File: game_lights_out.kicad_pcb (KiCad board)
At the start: 2 copper layers, 171.2 x 136.9 mm, 94 parts, among them SW1 SW_MEC_5E, SW10 SW_MEC_5E, SW11 SW_MEC_5E, SW12 SW_MEC_5E, SW13 SW_MEC_5E, SW14 SW_MEC_5E, SW15 SW_MEC_5E, SW16 SW_MEC_5E, SW17 SW_MEC_5E, SW18 SW_MEC_5E, SW19 SW_MEC_5E, SW2 SW_MEC_5E, SW20 SW_MEC_5E, SW21 SW_MEC_5E, SW22 SW_MEC_5E, SW23 SW_MEC_5E, SW24 SW_MEC_5E, SW25 SW_MEC_5E, SW26 SW_MEC_5E, SW27 SW_MEC_5E, SW28 SW_MEC_5E, SW29 SW_MEC_5E, SW3 SW_MEC_5E, SW30 SW_MEC_5E, SW31 SW_MEC_5E, SW32 SW_MEC_5E, SW33 SW_MEC_5E, SW34 SW_MEC_5E, SW35 SW_MEC_5E, SW36 SW_MEC_5E, SW37 SW_MEC_5E, SW38 SW_MEC_5E, SW39 SW_MEC_5E, SW4 SW_MEC_5E, SW40 SW_MEC_5E, SW5 SW_MEC_5E, SW6 SW_MEC_5E, SW7 SW_MEC_5E, SW8 SW_MEC_5E, SW9 SW_MEC_5E, U1 ATmega328-P, U2 ULN2803A

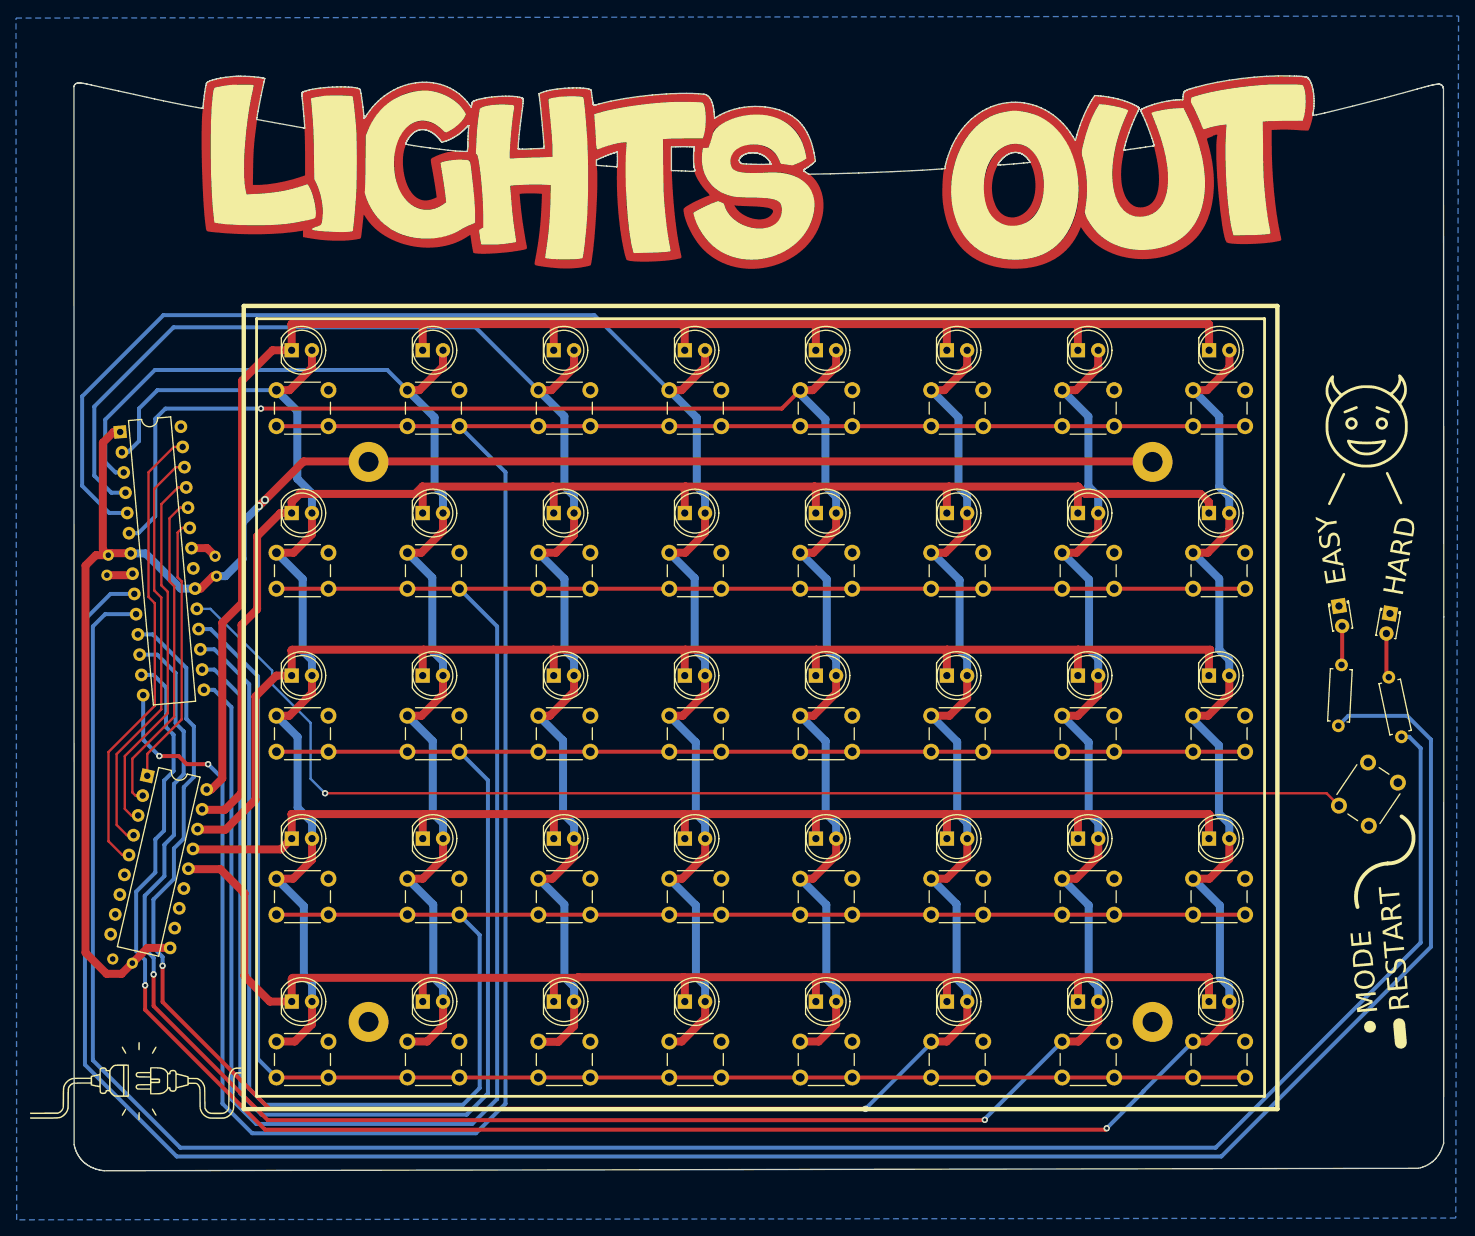
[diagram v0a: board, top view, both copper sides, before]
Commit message: Minor fixes in routing
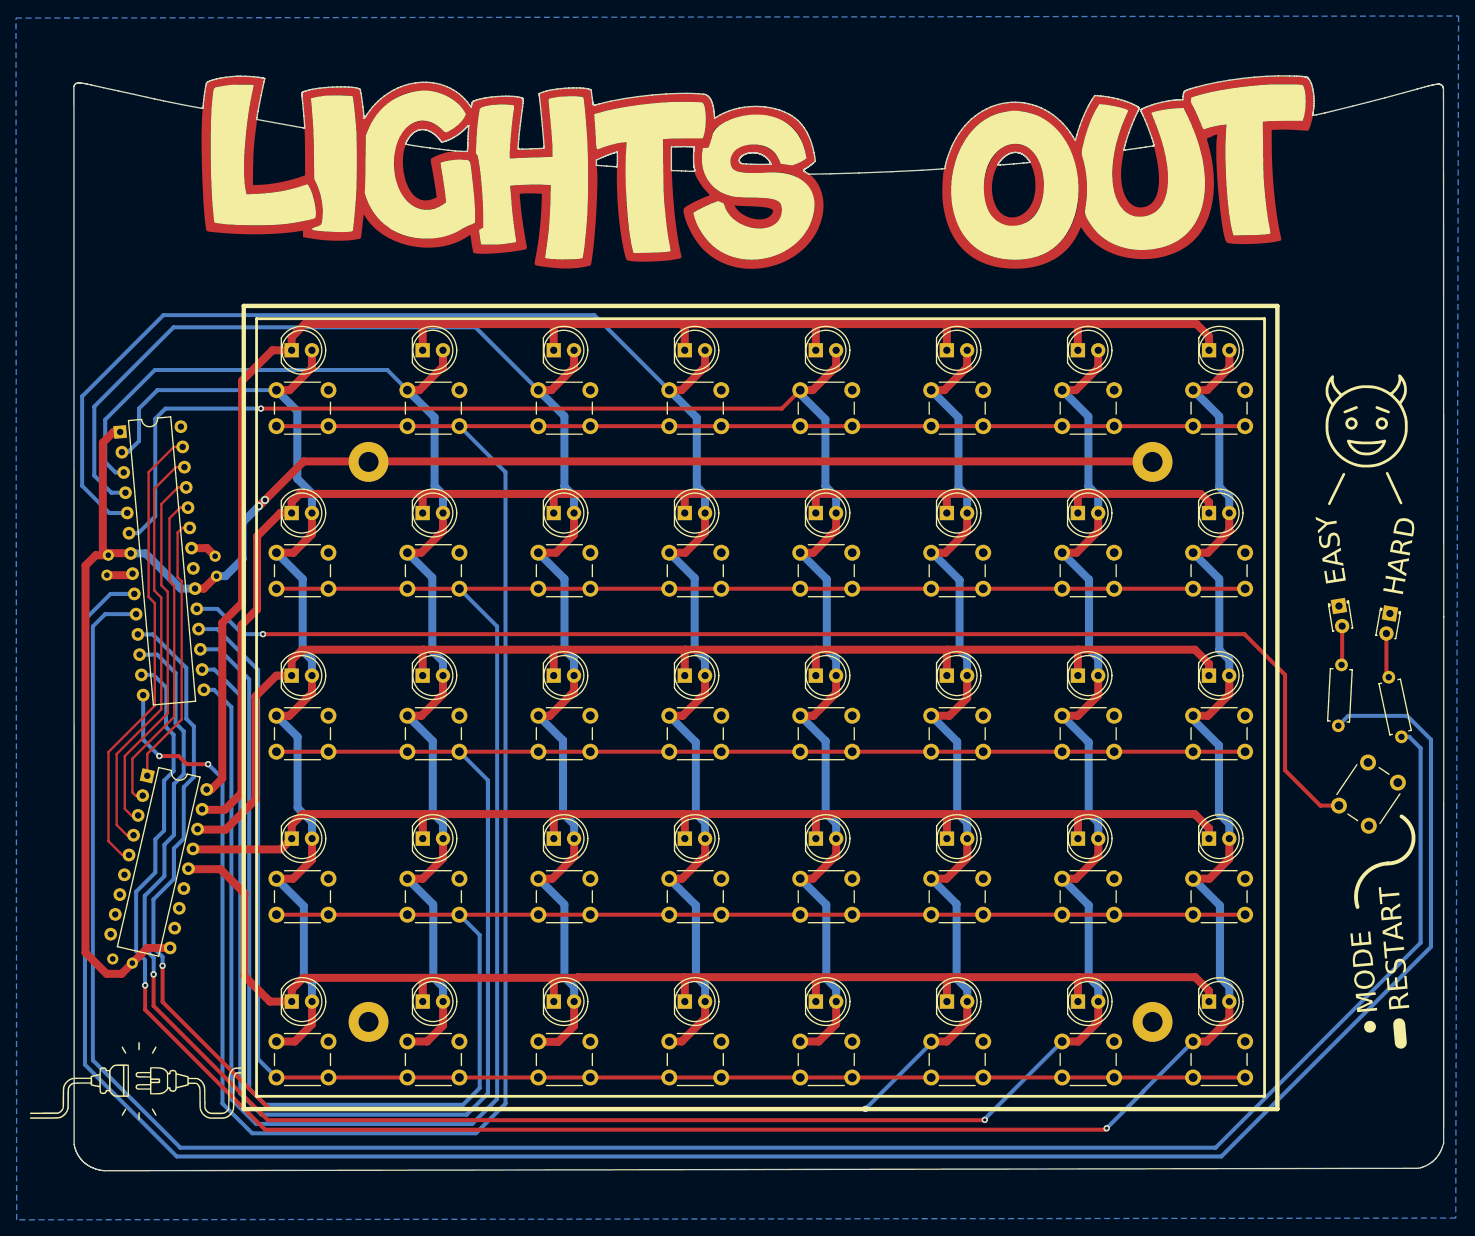
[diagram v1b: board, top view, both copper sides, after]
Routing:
- net R2: track 183.4 -> 176.9 mm
- net R3: track 168.3 -> 166.3 mm
- net R4: track 152.5 -> 150.6 mm
- net SCTL: track 158.4 -> 160.3 mm
- net R1: track 202.5 -> 200.6 mm
- net R5: track 165.1 -> 163.3 mm
